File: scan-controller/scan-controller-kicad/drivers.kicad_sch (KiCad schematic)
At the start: 56 parts, among them CN2 Motor, CN3 Fan, CN4 Lamp, Q1 CS12N06AE-G, U10 LGS5145, U11 MCP1416, U3 NH6375A50P, U4 DRV8871DDA, U6 TL431, U7 XL4015, U8 LM358

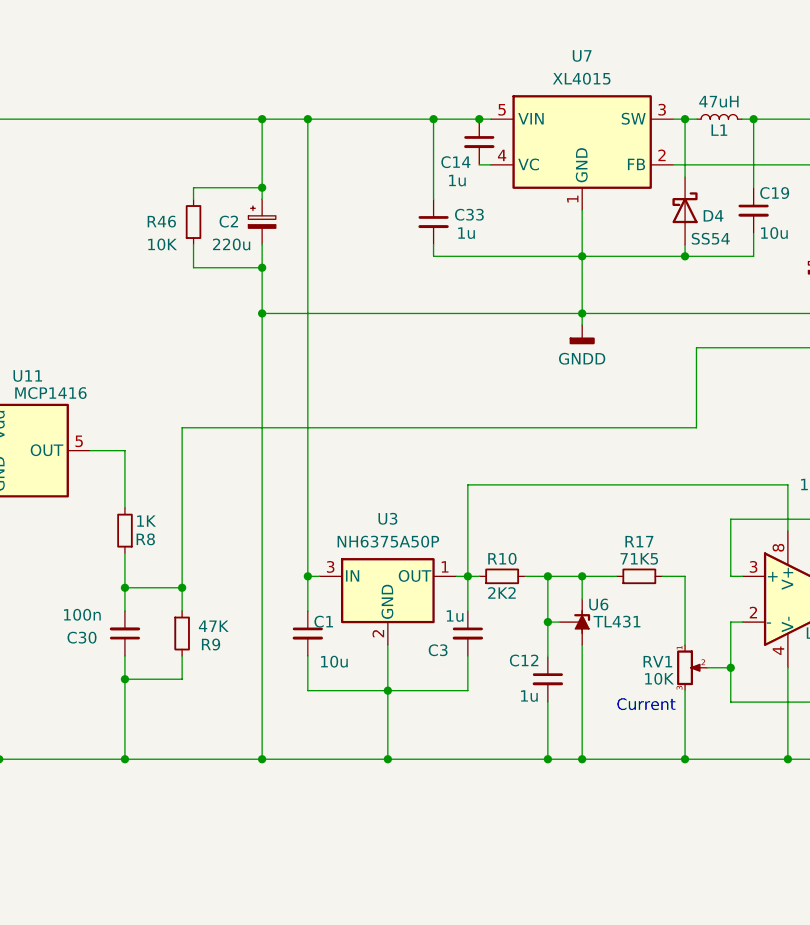
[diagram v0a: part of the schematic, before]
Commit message: DRC almost happy
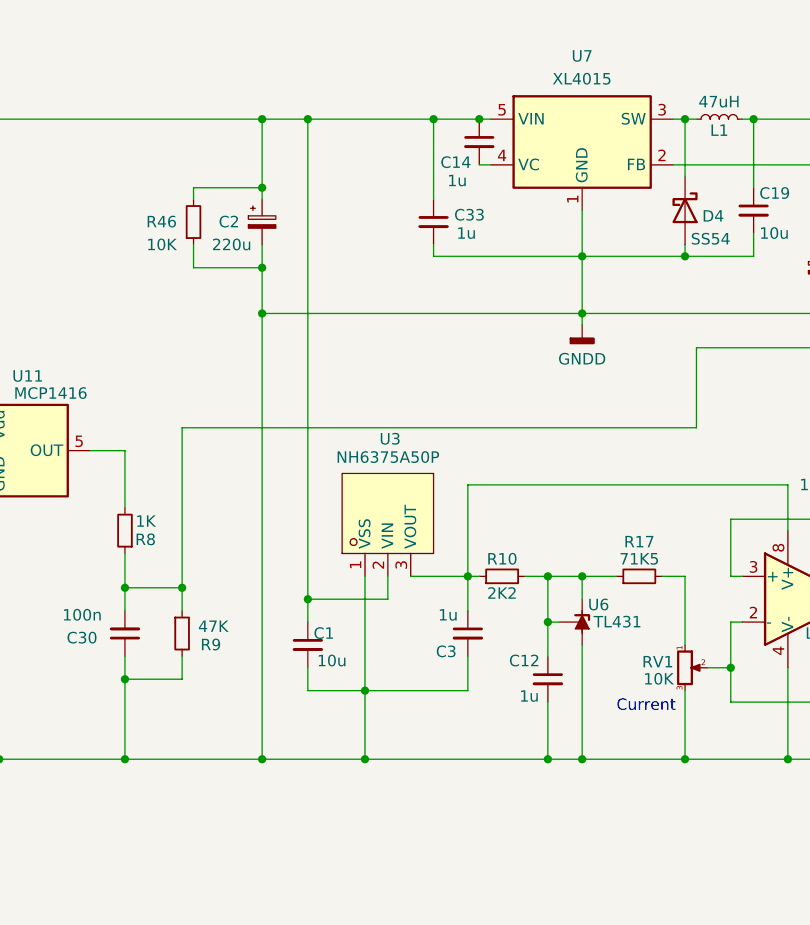
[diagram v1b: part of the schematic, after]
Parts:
- U3: footprint Package_TO_SOT_SMD:SOT-89-3 -> easyeda2kicad:SOT-89-3_L4.5-W2.5-P1.50-LS4.2-BR; symbol Regulator_Linear:L78L05_SOT89 -> easyeda2kicad:NH6375A50P; LCSC Part (none) -> C7427778
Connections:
- net 24VDC: now also U3.2 (VIN); no longer U3.3 (IN)
- net GNDD: now also U3.1 (VSS); no longer U3.2 (GND)
- net at C3.1, R10.1, U8.8 (V+): now also U3.3 (VOUT); no longer U3.1 (OUT)
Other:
- moved on the sheet: C1
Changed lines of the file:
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@@
 	)
 	(junction
+		(at 157.48 83.82)
+		(diameter 0)
+		(color 0 0 0 0)
+	)
+	(junction
 		(at 238.76 30.48)
 		(diameter 0)
@@
 	)
 	(junction
-		(at 166.37 93.98)
+		(at 163.83 93.98)
 		(diameter 0)
 		(color 0 0 0 0)
@@
 	)
 	(junction
+		(at 163.83 101.6)
+		(diameter 0)
+		(color 0 0 0 0)
+	)
+	(junction
 		(at 204.47 91.44)
 		(diameter 0)
@@
 	)
 	(junction
-		(at 166.37 101.6)
-		(diameter 0)
-		(color 0 0 0 0)
-	)
-	(junction
 		(at 93.98 180.34)
 		(diameter 0)
@@
 		(color 0 0 0 0)
 	)
-	(junction
-		(at 157.48 81.28)
-		(diameter 0)
-		(color 0 0 0 0)
-	)
 	(no_connect
 		(at 163.83 160.02)
@@
 	(wire
 		(pts
+			(xy 168.91 81.28) (xy 175.26 81.28)
+		)
+		(stroke
+			(width 0)
+			(type default)
+		)
+	)
+	(wire
+		(pts
 			(xy 158.75 157.48) (xy 163.83 157.48)
 		)
@@
 	(wire
 		(pts
-			(xy 157.48 90.17) (xy 157.48 93.98)
+			(xy 157.48 91.44) (xy 157.48 93.98)
 		)
 		(stroke
@@
 	(wire
 		(pts
-			(xy 152.4 101.6) (xy 166.37 101.6)
+			(xy 152.4 101.6) (xy 163.83 101.6)
 		)
 		(stroke
@@
 	(wire
 		(pts
+			(xy 163.83 93.98) (xy 175.26 93.98)
+		)
+		(stroke
+			(width 0)
+			(type default)
+		)
+	)
+	(wire
+		(pts
 			(xy 205.74 86.36) (xy 204.47 86.36)
 		)
@@
 	(wire
 		(pts
+			(xy 163.83 101.6) (xy 184.15 101.6)
+		)
+		(stroke
+			(width 0)
+			(type default)
+		)
+	)
+	(wire
+		(pts
 			(xy 276.86 58.42) (xy 276.86 62.23)
 		)
@@
 	(wire
 		(pts
-			(xy 157.48 30.48) (xy 157.48 81.28)
+			(xy 157.48 30.48) (xy 157.48 83.82)
 		)
 		(stroke
@@
 	(wire
 		(pts
-			(xy 166.37 93.98) (xy 175.26 93.98)
-		)
-		(stroke
-			(width 0)
-			(type default)
-		)
-	)
-	(wire
-		(pts
 			(xy 104.14 78.74) (xy 104.14 82.55)
 		)
@@
 	(wire
 		(pts
-			(xy 166.37 101.6) (xy 184.15 101.6)
+			(xy 187.96 101.6) (xy 199.39 101.6)
 		)
 		(stroke
@@
 	(wire
 		(pts
-			(xy 187.96 101.6) (xy 199.39 101.6)
+			(xy 43.18 101.6) (xy 43.18 99.06)
 		)
 		(stroke
@@
 	(wire
 		(pts
-			(xy 43.18 101.6) (xy 43.18 99.06)
+			(xy 104.14 67.31) (xy 104.14 73.66)
 		)
 		(stroke
@@
 	(wire
 		(pts
-			(xy 104.14 67.31) (xy 104.14 73.66)
+			(xy 163.83 81.28) (xy 163.83 93.98)
 		)
 		(stroke
@@
 	(wire
 		(pts
-			(xy 157.48 81.28) (xy 157.48 85.09)
-		)
-		(stroke
-			(width 0)
-			(type default)
-		)
-	)
-	(wire
-		(pts
 			(xy 49.53 88.9) (xy 49.53 93.98)
 		)
@@
 	(wire
 		(pts
-			(xy 157.48 93.98) (xy 166.37 93.98)
+			(xy 157.48 93.98) (xy 163.83 93.98)
 		)
 		(stroke
@@
 	(wire
 		(pts
-			(xy 157.48 81.28) (xy 158.75 81.28)
+			(xy 157.48 83.82) (xy 166.37 83.82)
 		)
 		(stroke
@@
 	(wire
 		(pts
-			(xy 173.99 81.28) (xy 175.26 81.28)
+			(xy 143.51 92.71) (xy 137.16 92.71)
 		)
 		(stroke
@@
 	(wire
 		(pts
-			(xy 143.51 92.71) (xy 137.16 92.71)
+			(xy 143.51 90.17) (xy 143.51 92.71)
 		)
 		(stroke
@@
 	(wire
 		(pts
-			(xy 143.51 90.17) (xy 143.51 92.71)
+			(xy 228.6 35.56) (xy 228.6 49.53)
 		)
 		(stroke
@@
 	(wire
 		(pts
-			(xy 228.6 35.56) (xy 228.6 49.53)
+			(xy 255.27 27.94) (xy 255.27 30.48)
 		)
 		(stroke
@@
 	(wire
 		(pts
-			(xy 255.27 27.94) (xy 255.27 30.48)
+			(xy 175.26 81.28) (xy 176.53 81.28)
 		)
 		(stroke
@@
 	(wire
 		(pts
-			(xy 175.26 81.28) (xy 176.53 81.28)
+			(xy 57.15 88.9) (xy 57.15 105.41)
 		)
 		(stroke
@@
 	(wire
 		(pts
-			(xy 57.15 88.9) (xy 57.15 105.41)
+			(xy 135.89 163.83) (xy 132.08 163.83)
 		)
 		(stroke
@@
 	(wire
 		(pts
-			(xy 135.89 163.83) (xy 132.08 163.83)
+			(xy 163.83 93.98) (xy 163.83 101.6)
 		)
 		(stroke
@@
 	(wire
 		(pts
+			(xy 166.37 83.82) (xy 166.37 81.28)
+		)
+		(stroke
+			(width 0)
+			(type default)
+		)
+	)
+	(wire
+		(pts
 			(xy 57.15 128.27) (xy 71.12 128.27)
 		)
@@
 	(wire
 		(pts
-			(xy 166.37 88.9) (xy 166.37 93.98)
+			(xy 196.85 81.28) (xy 199.39 81.28)
 		)
 		(stroke
@@
 	(wire
 		(pts
-			(xy 196.85 81.28) (xy 199.39 81.28)
+			(xy 264.16 46.99) (xy 264.16 49.53)
 		)
 		(stroke
@@
 	(wire
 		(pts
-			(xy 264.16 46.99) (xy 264.16 49.53)
+			(xy 204.47 74.93) (xy 264.16 74.93)
 		)
 		(stroke
@@
 	(wire
 		(pts
-			(xy 204.47 74.93) (xy 264.16 74.93)
+			(xy 210.82 71.12) (xy 210.82 76.2)
 		)
 		(stroke
@@
 	(wire
 		(pts
-			(xy 210.82 71.12) (xy 210.82 76.2)
+			(xy 176.53 35.56) (xy 177.8 35.56)
 		)
 		(stroke
@@
 	(wire
 		(pts
-			(xy 176.53 35.56) (xy 177.8 35.56)
+			(xy 74.93 153.67) (xy 85.09 153.67)
 		)
 		(stroke
@@
 	(wire
 		(pts
-			(xy 74.93 153.67) (xy 85.09 153.67)
+			(xy 123.19 101.6) (xy 137.16 101.6)
 		)
 		(stroke
@@
 	(wire
 		(pts
-			(xy 123.19 101.6) (xy 137.16 101.6)
+			(xy 157.48 83.82) (xy 157.48 86.36)
 		)
 		(stroke
@@
 	(wire
 		(pts
-			(xy 166.37 93.98) (xy 166.37 101.6)
-		)
-		(stroke
-			(width 0)
-			(type default)
-		)
-	)
-	(wire
-		(pts
 			(xy 198.12 30.48) (xy 199.39 30.48)
 		)
@@
 	(symbol
 		(lib_id "Device:C_Small")
-		(at 157.48 87.63 0)
+		(at 157.48 88.9 0)
 		(unit 1)
 		(exclude_from_sim no)
@@
 		(dnp no)
 		(property "Reference" "C1"
-			(at 158.115 86.36 0)
+			(at 158.115 87.63 0)
 			(effects
 				(font
@@
 		)
 		(property "Value" "10u"
-			(at 158.75 90.805 0)
+			(at 158.496 90.678 0)
 			(effects
 				(font
@@
 		)
 		(property "Footprint" "Capacitor_SMD:C_1210_3225Metric"
-			(at 157.48 87.63 0)
+			(at 157.48 88.9 0)
 			(effects
 				(font
@@
 		)
 		(property "Datasheet" "https://datasheet.lcsc.com/lcsc/2209061730_PSA-Prosperity-Dielectrics-FS32X106K101EGG_C5156756.pdf"
-			(at 157.48 87.63 0)
+			(at 157.48 88.9 0)
 			(effects
 				(font
@@
 		)
 		(property "Description" "10u 100V X7R"
-			(at 157.48 87.63 0)
+			(at 157.48 88.9 0)
 			(effects
 				(font
@@
 		)
 		(property "LCSC" "C5156756"
-			(at 157.48 87.63 0)
+			(at 157.48 88.9 0)
 			(effects
 				(font
@@
 		)
 		(property "Inventory" "B"
-			(at 157.48 87.63 0)
+			(at 157.48 88.9 0)
 			(effects
 				(font
@@
 			)
 		)
-		(property "Description" "Resistor, small symbol"
+		(property "Description" "1W 200V 50mΩ 1%"
 			(at 264.16 88.9 0)
 			(effects
@@
 	)
 	(symbol
-		(lib_id "Regulator_Linear:L78L05_SOT89")
-		(at 166.37 81.28 0)
+		(lib_id "easyeda2kicad:NH6375A50P")
+		(at 166.37 73.66 90)
 		(unit 1)
 		(exclude_from_sim no)
@@
 		(dnp no)
 		(property "Reference" "U3"
-			(at 166.37 74.93 0)
+			(at 166.624 66.04 90)
 			(effects
 				(font
@@
 		)
 		(property "Value" "NH6375A50P"
-			(at 166.37 77.47 0)
+			(at 166.37 68.072 90)
 			(effects
 				(font
@@
 			)
 		)
-		(property "Footprint" "Package_TO_SOT_SMD:SOT-89-3"
-			(at 166.37 76.2 0)
+		(property "Footprint" "easyeda2kicad:SOT-89-3_L4.5-W2.5-P1.50-LS4.2-BR"
+			(at 176.53 73.66 0)
 			(effects
 				(font
 					(size 1.27 1.27)
-					(italic yes)
 				)
 				(hide yes)
@@
 		)
 		(property "Datasheet" "https://jlcpcb.com/api/file/downloadByFileSystemAccessId/8602998189351972864"
-			(at 166.37 82.55 0)
+			(at 166.37 73.66 0)
 			(effects
 				(font
@@
 		)
 		(property "Description" "50V 5V LDO"
-			(at 166.37 81.28 0)
+			(at 166.37 73.66 0)
 			(effects
 				(font
@@
 		)
 		(property "Inventory" "B"
-			(at 166.37 81.28 0)
+			(at 166.37 73.66 0)
 			(effects
 				(font
@@
 		)
 		(property "LCSC" "C7427778"
-			(at 166.37 81.28 0)
+			(at 166.37 73.66 0)
+			(effects
+				(font
+					(size 1.27 1.27)
+				)
+				(hide yes)
+			)
+		)
+		(property "LCSC Part" "C7427778"
+			(at 179.07 73.66 0)
 			(effects
 				(font
@@
 		(dnp no)
 		(property "Reference" "C3"
-			(at 170.815 89.535 0)
+			(at 171.704 89.662 0)
 			(effects
 				(font
@@
 		)
 		(property "Value" "1u"
-			(at 172.72 85.725 0)
+			(at 171.958 85.598 0)
 			(effects
 				(font
